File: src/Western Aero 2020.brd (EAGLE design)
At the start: 122.2 x 99.4 mm, 85 parts

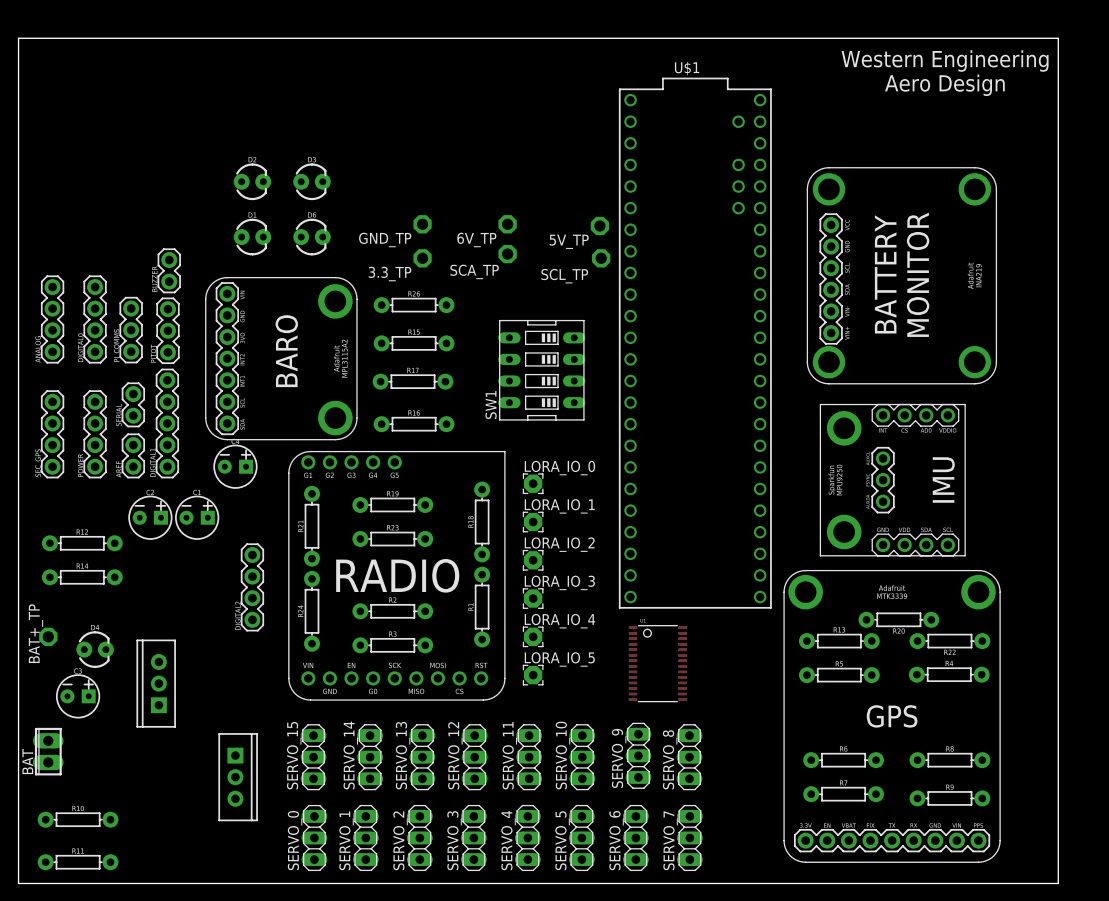
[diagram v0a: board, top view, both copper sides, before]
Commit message: new layout
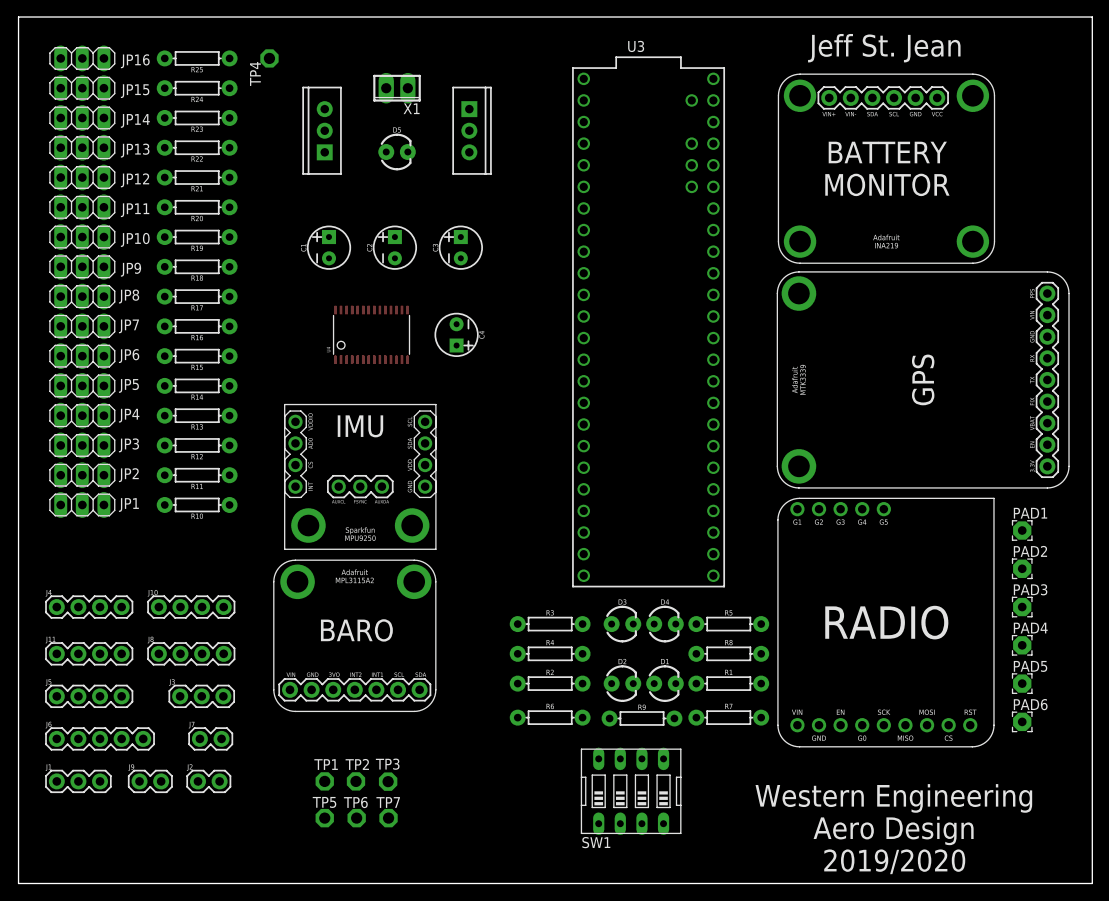
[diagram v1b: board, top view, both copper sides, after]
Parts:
- removed 3.3_TP, 5V_TP, 6V_TP, BAT+_TP, GND_TP, SCA_TP, SCL_TP: PTR1PAD1-13, testpad:P1-13
- removed 7805, 7806: (no value), SparkFun-IC-Power:TO220-IGO
- removed ANALOG, DIGITAL0, DIGITAL2, POWER, SEC_GPS: (no value), SparkFun-Connectors:1X04
- removed AREF, BUZZER, SERIAL: (no value), SparkFun-Connectors:1X02
- removed BAT: (no value), con-phoenix-254:2POL254
- removed D6: Red, SparkFun-LED:LED_3MM
- removed DIGITAL1: (no value), SparkFun-Connectors:1X05
- removed LORA_IO_0, LORA_IO_1, LORA_IO_2, LORA_IO_3, LORA_IO_4, LORA_IO_5: WIREPAD, wirepad:2,15/1,0
- removed PITOT, PI_COMMS: (no value), SparkFun-Connectors:1X03
- removed R26: 10K, SparkFun-Resistors:AXIAL-0.3
- removed SERVO_0, SERVO_1, SERVO_10, SERVO_11, SERVO_12, SERVO_13, SERVO_14, SERVO_15, SERVO_2, SERVO_3, SERVO_4, SERVO_5, SERVO_6, SERVO_7, SERVO_8, SERVO_9: (no value), pinhead:1X03
- removed U$1: TEENSY_3.5_DIL+4, Teensy_3_and_LC_Series_Boards_v1.4:TEENSY_3.5_DIL+4
- removed U$2: SPARKFUN_MPU9250_IMU, AERO_Eagle_Library:SPARKFUN_MPU9250_IMU
- removed U$3: ADAFRUIT_RFM95W_LORA_RADIO, AERO_Eagle_Library:ADAFRUIT_RFM95W_LORA_RADIO
- removed U$4: ADAFRUIT_MPL3115A2_BAROMETER, AERO_Eagle_Library:ADAFRUIT_MPL3115A2_BAROMETER
- removed U$5: ADAFRUIT_INA219_BATTERY_SENSOR, AERO_Eagle_Library:ADAFRUIT_INA219_BATTERY_SENSOR
- removed U$6: ADAFRUIT_MTK3339_GPS, AERO_Eagle_Library:ADAFRUIT_MTK3339_GPS
- added D5: Green, SparkFun-LED:LED_3MM
- added J1, J3: (no value), SparkFun-Connectors:1X03
- added J10, J11, J4, J5, J8: (no value), SparkFun-Connectors:1X04
- added J2, J7, J9: (no value), SparkFun-Connectors:1X02
- added J6: (no value), SparkFun-Connectors:1X05
- added JP1, JP10, JP11, JP12, JP13, JP14, JP15, JP16, JP2, JP3, JP4, JP5, JP6, JP7, JP8, JP9: (no value), pinhead:1X03
- added PAD1, PAD2, PAD3, PAD4, PAD5, PAD6: WIREPAD, wirepad:2,15/1,0
- added R25: 220, SparkFun-Resistors:AXIAL-0.3
- added TP1, TP2, TP3, TP4, TP5, TP6, TP7: PTR1PAD1-13, testpad:P1-13
- added U2: 7805, SparkFun-IC-Power:TO220-IGO
- added U3: TEENSY_3.5_DIL+4, Teensy_3_and_LC_Series_Boards_v1.4:TEENSY_3.5_DIL+4
- added U4: (no value), adafruit:TSSOP28
- added U5: SPARKFUN_MPU9250_IMU, AERO_Eagle_Library:SPARKFUN_MPU9250_IMU
- added U6: ADAFRUIT_MPL3115A2_BAROMETER, AERO_Eagle_Library:ADAFRUIT_MPL3115A2_BAROMETER
- added U7: ADAFRUIT_INA219_BATTERY_SENSOR, AERO_Eagle_Library:ADAFRUIT_INA219_BATTERY_SENSOR
- added U8: ADAFRUIT_RFM95W_LORA_RADIO, AERO_Eagle_Library:ADAFRUIT_RFM95W_LORA_RADIO
- added U9: ADAFRUIT_MTK3339_GPS, AERO_Eagle_Library:ADAFRUIT_MTK3339_GPS
- added X1: (no value), con-phoenix-254:2POL254
- C1: value 10uF -> 0.1uF
- C2: value 0.1uF -> 0.33uF
- C3: value 0.33uF -> 0.1uF
- C4: value 0.1uF -> 10uF
- D1: value Blue -> Red
- D2: value Yellow -> Blue
- D3: value White -> Yellow
- D4: value Green -> White
- R15, R16, R17: value 10K -> 220
- R6, R7, R8, R9: value 220 -> 10K
- U1: value (none) -> 7806; device adafruit:TSSOP28 -> SparkFun-IC-Power:TO220-IGO
- moved R22 105.8 mm to (21.0, 86.5)
- moved R20 95.7 mm to (21.0, 79.5)
- moved R13 80.0 mm to (21.0, 55.0), turned to 180 degrees
- moved U1 73.9 mm to (36.0, 88.5), turned to 90 degrees
- moved D2 73.3 mm to (71.0, 23.5)
- moved D1 71.5 mm to (76.0, 23.5)
- moved C3 69.3 mm to (52.0, 74.8), turned to 90 degrees
- moved D4 67.1 mm to (76.0, 30.5)
- moved D3 63.5 mm to (71.0, 30.5)
- moved R24 63.0 mm to (21.0, 93.5), turned to 180 degrees
- moved R23 54.6 mm to (21.0, 90.0), turned to 180 degrees
- moved SW1 50.6 mm to (72.0, 10.8), turned to 0 degrees
- moved R11 47.6 mm to (21.0, 48.0), turned to 180 degrees
- moved R4 47.0 mm to (62.5, 27.0)
- moved R18 45.0 mm to (21.0, 72.5), turned to 180 degrees
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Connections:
- net 3.3V: now also J11.2, TP7.TP, U3.3.3V, U3.3.3V3, U5.VDD; no longer 3.3_TP.TP, POWER.2, U$1.3.3V, U$1.3.3V3, U$2.VDD
- net 5V: now also C3.1, D5.A, J1.2, J11.1, J4.2, TP6.TP, U2.OUT, U3.VIN, U4.1, U4.2, U4.28, U4.3, U6.VIN, U7.VCC, U8.1, U9.VIN; no longer 5V_TP.TP, 7805.OUT, C1.1, D4.A, PITOT.2, POWER.1, SEC_GPS.2, U$1.VIN, U$3.1, U$4.VIN, U$5.VCC, U$6.VIN, U1.1, U1.2, U1.28, U1.3
- net 6V: now also C1.1, JP1.2, JP10.2, JP11.2, JP12.2, JP13.2, JP14.2, JP15.2, JP16.2, JP2.2, JP3.2, JP4.2, JP5.2, JP6.2, JP7.2, JP8.2, JP9.2, TP1.TP, U1.OUT; no longer 6V_TP.TP, 7806.OUT, C2.1, SERVO_0.2, SERVO_1.2, SERVO_10.2, SERVO_11.2, SERVO_12.2, SERVO_13.2, SERVO_14.2, SERVO_15.2, SERVO_2.2, SERVO_3.2, SERVO_4.2, SERVO_5.2, SERVO_6.2, SERVO_7.2, SERVO_8.2, SERVO_9.2
- net A10: now also J10.1, U3.A10; no longer ANALOG.1, U$1.A10
- net A11: now also J10.2, U3.A11; no longer ANALOG.2, U$1.A11
- net A21: now also J10.3, U3.A21; no longer ANALOG.3, U$1.A21
- net A22: now also J10.4, U3.A22; no longer ANALOG.4, U$1.A22
- net AGND: now also J9.1, U3.AGND; no longer AREF.1, U$1.AGND
- net AREF: now also J9.2, U3.AREF; no longer AREF.2, U$1.AREF
- net BLUE_LED: now also D2.A, U3.21/A7; no longer D1.A, U$1.21/A7
- net BUZZER: now also J2.1, U3.2; no longer BUZZER.1, U$1.2
- net CS: now also J5.4, U3.33/A14, U8.8; no longer DIGITAL2.4, U$1.33/A14, U$3.8
- net D3: now also J8.1, U3.3; no longer DIGITAL0.1, U$1.3
- net D35: now also J6.1, U3.35/A16; no longer DIGITAL1.1, U$1.35/A16
- net D36: now also J6.2, U3.36/A17; no longer DIGITAL1.2, U$1.36/A17
- net D37: now also J6.3, U3.37/A18; no longer DIGITAL1.3, U$1.37/A18
- net D38: now also J6.4, U3.38/A19; no longer DIGITAL1.4, U$1.38/A19
- net D39: now also J6.5, U3.39/A20; no longer DIGITAL1.5, U$1.39/A20
- net D4: now also J8.2, U3.4; no longer DIGITAL0.2, U$1.4
- net D5: now also J8.3, U3.5; no longer DIGITAL0.3, U$1.5
- net D6: now also J8.4, U3.6; no longer DIGITAL0.4, U$1.6
- net DIP1: now also R6.P$2, U3.24; no longer R26.P$2, U$1.24
- net DIP2: now also R7.P$2, U3.25; no longer R15.P$2, U$1.25
- net DIP3: now also R8.P$2, U3.26; no longer R16.P$2, U$1.26
- net DIP4: now also R9.P$2, U3.27; no longer R17.P$2, U$1.27
- net ENV_INT1: now also U3.29, U6.INT1; no longer U$1.29, U$4.INT1
- net ENV_INT2: now also U3.30, U6.INT2; no longer U$1.30, U$4.INT2
- net GND: now also J1.1, J11.4, J2.2, J3.1, J4.1, JP1.3, JP10.3, JP11.3, JP12.3, JP13.3, JP14.3, JP15.3, JP16.3, JP2.3, JP3.3, JP4.3, JP5.3, JP6.3, JP7.3, JP8.3, JP9.3, R1.P$1, R2.P$1, R3.P$1, R4.P$1, R5.P$1, R6.P$1, R7.P$1, R8.P$1, R9.P$1, TP2.TP, U1.GND, U2.GND, U3.GND, U3.GND1, U4.14, U4.23, U4.24, U4.25, U4.4, U4.5, U5.AD0, U5.FSYNC, U5.GND, U6.GND, U7.GND, U8.2, U9.GND, X1.1; no longer 7805.GND, 7806.GND, BAT.1, BUZZER.2, GND_TP.TP, PITOT.1, PI_COMMS.1, POWER.4, R10.P$1, R11.P$1, R12.P$1, R13.P$1, R14.P$1, R15.P$1, R16.P$1, R17.P$1, R26.P$1, SEC_GPS.1, SERVO_0.3, SERVO_1.3, SERVO_10.3, SERVO_11.3, SERVO_12.3, SERVO_13.3, SERVO_14.3, SERVO_15.3, SERVO_2.3, SERVO_3.3, SERVO_4.3, SERVO_5.3, SERVO_6.3, SERVO_7.3, SERVO_8.3, SERVO_9.3, U$1.GND, U$1.GND1, U$2.AD0, U$2.FSYNC, U$2.GND, U$3.2, U$4.GND, U$5.GND, U$6.GND, U1.14, U1.23, U1.24, U1.25, U1.4, U1.5
- net GPS_EN: now also U3.15/A1, U9.EN; no longer U$1.15/A1, U$6.EN
- net GPS_FIX: now also U3.16/A2, U9.FIX; no longer U$1.16/A2, U$6.FIX
- net GPS_PPS: now also U3.17/A3, U9.PPS; no longer U$1.17/A3, U$6.PPS
- net IMU_INT: now also U3.28, U5.INT; no longer U$1.28, U$2.INT
- net LORA_EN: now also U3.32/A13, U8.3; no longer U$1.32/A13, U$3.3
- net LORA_INT: now also U3.31/A12; no longer U$1.31/A12
- net LORA_RST: now also U3.34/A15, U8.9; no longer U$1.34/A15, U$3.9
- net MISO: now also J5.2, U3.12, U8.6; no longer DIGITAL2.2, U$1.12, U$3.6
- net MOSI: now also J5.3, U3.11, U8.7; no longer DIGITAL2.3, U$1.11, U$3.7
- net N$1: now also JP1.1, R10.P$2; no longer R18.P$2, SERVO_0.1
- net N$10: now also PAD3.1, U8.11; no longer LORA_IO_2.1, U$3.11
- net N$11: now also JP3.1, R12.P$2; no longer R2.P$2, SERVO_2.1
- net N$12: now also JP4.1, R13.P$2; no longer R3.P$2, SERVO_3.1
- net N$13: now also JP5.1, R14.P$2; no longer R4.P$2, SERVO_4.1
- net N$14: now also JP6.1, R15.P$2; no longer R5.P$2, SERVO_5.1
- net N$15: now also JP7.1, R16.P$2; no longer R6.P$2, SERVO_6.1
- net N$16: now also JP8.1, R17.P$2; no longer R7.P$2, SERVO_7.1
- net N$17: now also JP9.1, R18.P$2; no longer R8.P$2, SERVO_8.1
- net N$18: now also JP10.1, R19.P$2; no longer R9.P$2, SERVO_9.1
- net N$19: now also JP11.1, R20.P$2; no longer R19.P$2, SERVO_10.1
- net N$2: now also D1.K, R1.P$2; no longer D6.K, R10.P$2
- net N$20: now also JP12.1, R21.P$2; no longer R20.P$2, SERVO_11.1
- net N$21: now also JP13.1, R22.P$2; no longer R21.P$2, SERVO_12.1
- net N$22: now also JP14.1, R23.P$2; no longer R22.P$2, SERVO_13.1
- net N$23: now also JP15.1, R24.P$2; no longer R23.P$2, SERVO_14.1
- net N$24: now also JP16.1, R25.P$2; no longer R24.P$2, SERVO_15.1
- net N$25: now also PAD5.1, U8.13; no longer LORA_IO_4.1, U$3.13
- net N$26: now also PAD4.1, U8.12; no longer LORA_IO_3.1, U$3.12
- net N$27: now also PAD1.1, U8.4; no longer LORA_IO_0.1, U$3.4
- net N$3: now also D2.K, R2.P$2; no longer D1.K, R11.P$2
- net N$4: now also D3.K, R3.P$2; no longer D2.K, R12.P$2
- net N$5: now also D4.K, R5.P$2; no longer D3.K, R13.P$2
- net N$6: now also D5.K, R4.P$2; no longer D4.K, R14.P$2
- net N$7: now also PAD6.1, U8.14; no longer LORA_IO_5.1, U$3.14
- net N$8: now also PAD2.1, U8.10; no longer LORA_IO_1.1, U$3.10
- net N$9: now also JP2.1, R11.P$2; no longer R1.P$2, SERVO_1.1
- net PITOT: now also J1.3, U3.14/A0; no longer PITOT.3, U$1.14/A0
- net PWM0: now also R10.P$1, U4.6; no longer R18.P$1, U1.6
- net PWM1: now also R11.P$1, U4.7; no longer R1.P$1, U1.7
- net PWM10: now also R20.P$1, U4.17; no longer R19.P$1, U1.17
- net PWM11: now also R21.P$1, U4.18; no longer R20.P$1, U1.18
- net PWM12: now also R22.P$1, U4.19; no longer R21.P$1, U1.19
- net PWM13: now also R23.P$1, U4.20; no longer R22.P$1, U1.20
- net PWM14: now also R24.P$1, U4.21; no longer R23.P$1, U1.21
- net PWM15: now also R25.P$1, U4.22; no longer R24.P$1, U1.22
- net PWM2: now also R12.P$1, U4.8; no longer R2.P$1, U1.8
- net PWM3: now also R13.P$1, U4.9; no longer R3.P$1, U1.9
- net PWM4: now also R14.P$1, U4.10; no longer R4.P$1, U1.10
- net PWM5: now also R15.P$1, U4.11; no longer R5.P$1, U1.11
- net PWM6: now also R16.P$1, U4.12; no longer R6.P$1, U1.12
- net PWM7: now also R17.P$1, U4.13; no longer R7.P$1, U1.13
- net PWM8: now also R18.P$1, U4.15; no longer R8.P$1, U1.15
- net PWM9: now also R19.P$1, U4.16; no longer R9.P$1, U1.16
- net RED_LED: now also D1.A, U3.20/A6; no longer D6.A, U$1.20/A6
- net RX1: now also J7.1, U3.0; no longer SERIAL.1, U$1.0
- net RX2: now also J3.3, U3.9; no longer PI_COMMS.3, U$1.9
- net RX3: now also J4.4, U3.7, U9.RX; no longer SEC_GPS.4, U$1.7, U$6.RX
- net SCK: now also J5.1, U3.13, U8.5; no longer DIGITAL2.1, U$1.13, U$3.5
- net SCL: now also TP3.TP, U3.19/A5, U4.26, U5.SCL, U6.SCL, U7.SCL; no longer SCL_TP.TP, U$1.19/A5, U$2.SCL, U$4.SCL, U$5.SCL, U1.26
- net SDA: now also TP5.TP, U3.18/A4, U4.27, U5.SDA, U6.SDA, U7.SDA; no longer SCA_TP.TP, U$1.18/A4, U$2.SDA, U$4.SDA, U$5.SDA, U1.27
- net TX1: now also J7.2, U3.1; no longer SERIAL.2, U$1.1
- net TX2: now also J3.2, U3.10; no longer PI_COMMS.2, U$1.10
- net TX3: now also J4.3, U3.8, U9.TX; no longer SEC_GPS.3, U$1.8, U$6.TX
- net VIN+: now also TP4.TP, U7.VIN+, X1.2; no longer BAT+_TP.TP, BAT.2, U$5.VIN+
- net VIN-: now also C2.1, U1.IN, U2.IN, U7.VIN-; no longer 7805.IN, 7806.IN, C3.1, U$5.VIN-
- net VUSB: now also J11.3, U3.VUSB; no longer POWER.3, U$1.VUSB
- net WHITE_LED: now also D4.A, U3.23/A9; no longer D3.A, U$1.23/A9
- net YELLOW_LED: now also D3.A, U3.22/A8; no longer D2.A, U$1.22/A8
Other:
- board size 122.2 x 99.4 mm -> 126.2 x 101.9 mm
- board text added: "Jeff St. Jean"
- board text added: "Western Engineering Aero Design 2019/2020"
- board text removed: "Western Engineering Aero Design"
